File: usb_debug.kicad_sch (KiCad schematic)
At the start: 40 parts, among them IC3 93LC66BT-I_MC, J1 USB_C_Receptacle_USB2.0, J5 USB_C_Receptacle_USB2.0, U1 MIMXRT1052CVJ5B, U5 FT2232HQ, U7 PRTR5V0U2X, Y3 830105420809

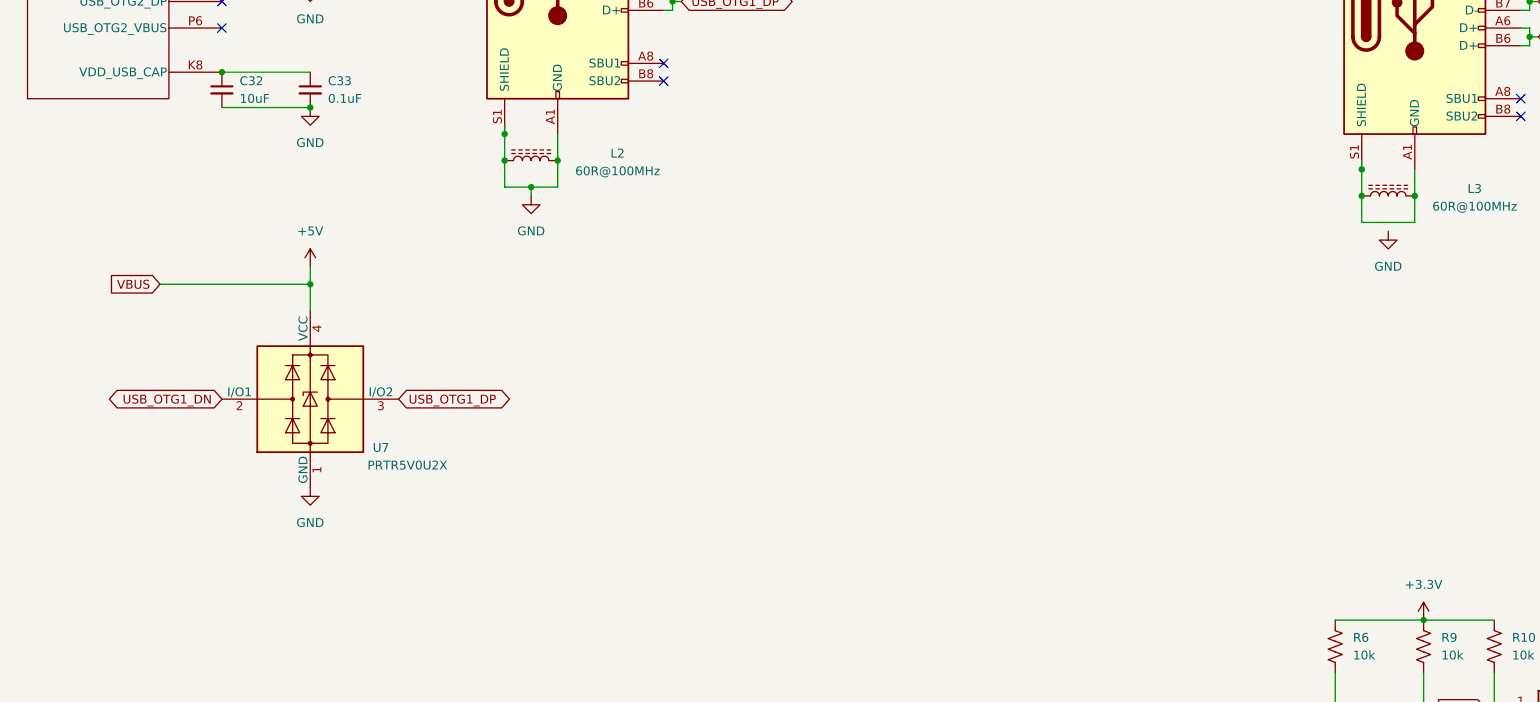
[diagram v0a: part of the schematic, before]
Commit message: finished layout of v0.2!
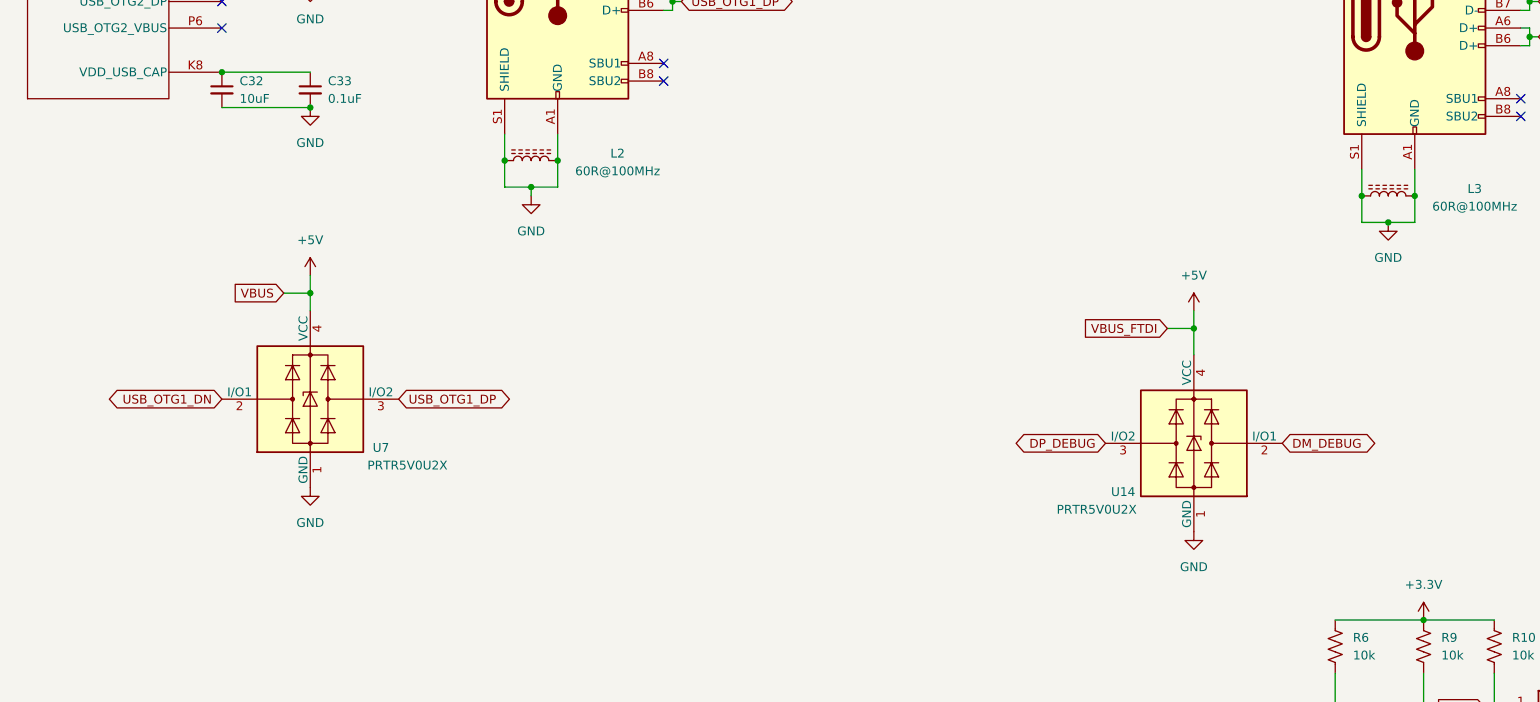
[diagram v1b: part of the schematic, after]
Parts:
- added U14: PRTR5V0U2X, Package_TO_SOT_SMD:SOT-143, symbol Power_Protection:PRTR5V0U2X
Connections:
- net VBUS_FTDI is gone; now on net +5V: CR2.2
- net +5V: now also U14.4 (VCC)
- net DM_DEBUG: now also U14.2 (I/O1)
- net DP_DEBUG: now also U14.3 (I/O2)
- net GND: now also J1.A1 (GND), J1.A12 (GND), J1.B1 (GND), J1.B12 (GND), J1.S1 (SHIELD), L3.1, L3.2, U14.1 (GND)
